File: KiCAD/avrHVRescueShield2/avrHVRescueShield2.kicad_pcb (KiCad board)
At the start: 2 copper layers, 68.6 x 53.3 mm, 24 parts, among them Q1 MUN5311DW1T1G, SW1 SW_Push, U1 ATmega328P-PU, U2 ATtiny85-20PU, U3 ATtiny2313-20PU, U4 MC34063AP

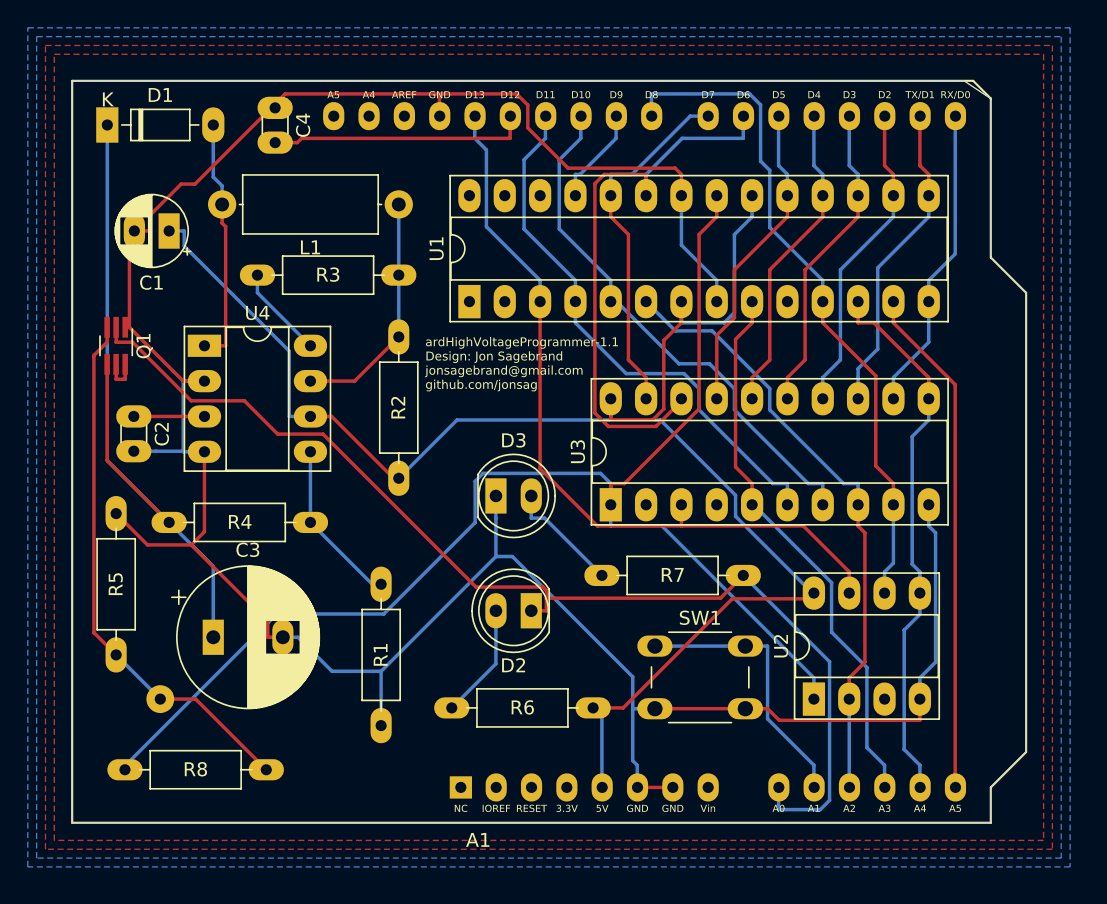
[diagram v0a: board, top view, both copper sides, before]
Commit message: new pcb
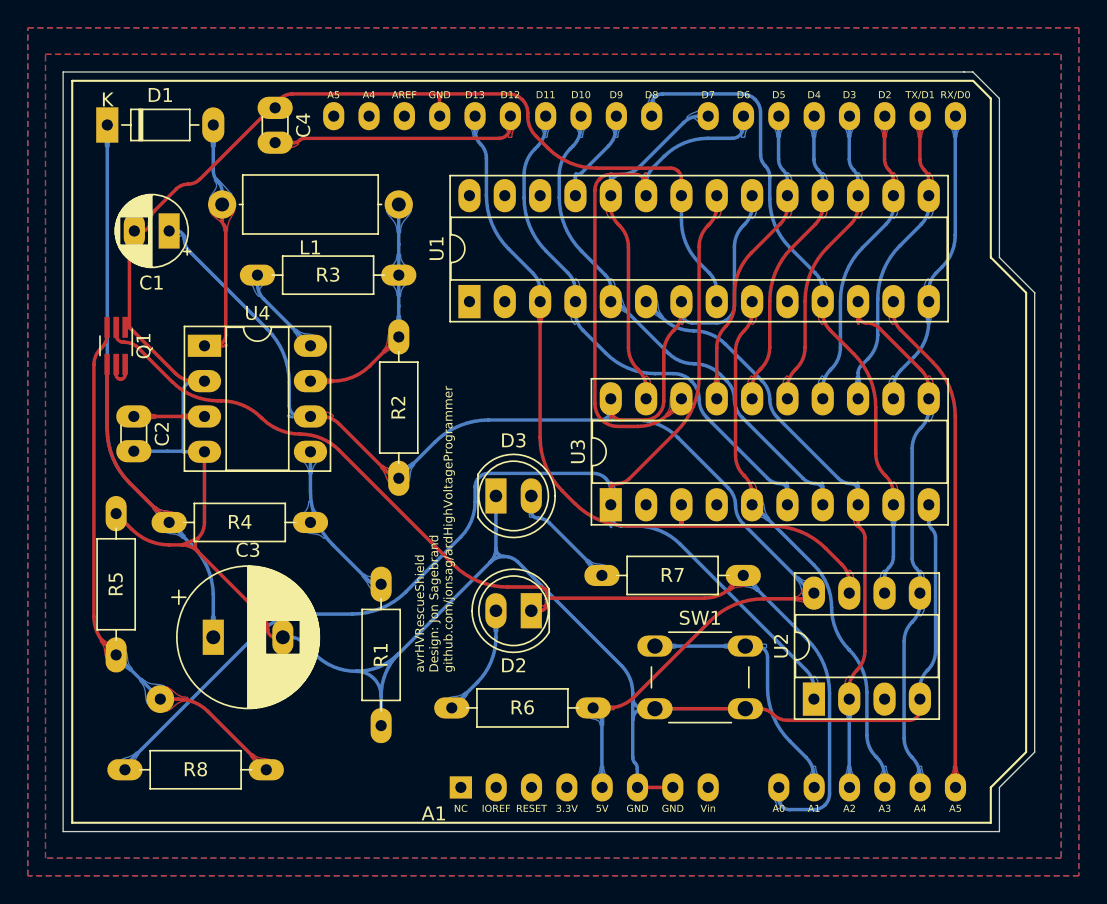
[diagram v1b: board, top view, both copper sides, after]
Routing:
- net GND: track 198.2 -> 203.6 mm
- net 12V_EN: track 81.0 -> 78.6 mm
- net ~{RESET}: track 95.6 -> 93.3 mm
- net +5V: track 120.2 -> 118.2 mm
- net XA0: track 49.1 -> 47.5 mm
- net ~{OE}: track 39.5 -> 38.0 mm
- net DATA6: track 40.7 -> 39.2 mm
- net RDY: track 55.6 -> 54.4 mm
- net XTAL1: track 39.9 -> 38.7 mm
- net XA1: track 39.4 -> 38.3 mm
- net BS1: track 44.1 -> 43.0 mm
- net DATA7: track 25.9 -> 25.0 mm
- net ~{WR}: track 38.8 -> 37.9 mm
- net +12V: track 53.2 -> 52.4 mm
- net ~{GO}: track 19.6 -> 18.9 mm
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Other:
- board size 68.6 x 53.3 mm -> 69.8 x 54.6 mm
- board text added: "avrHVRescueShield Design: Jon Sagebrand github.com/jonsag/ardHighVoltageProgrammer"
- board text removed: "ardHighVoltageProgrammer-1.1 Design: Jon Sagebrand jonsagebrand@gmail.com github.com/jonsag"
